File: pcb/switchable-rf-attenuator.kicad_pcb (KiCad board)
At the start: 4 copper layers, 47.4 x 31.5 mm, 26 parts, among them J1 USB_B_Mini, J2 Conn_Coaxial, J3 Conn_Coaxial, SW1 SW_SPDT, U1 AS183-73LF, U2 AS183-73LF

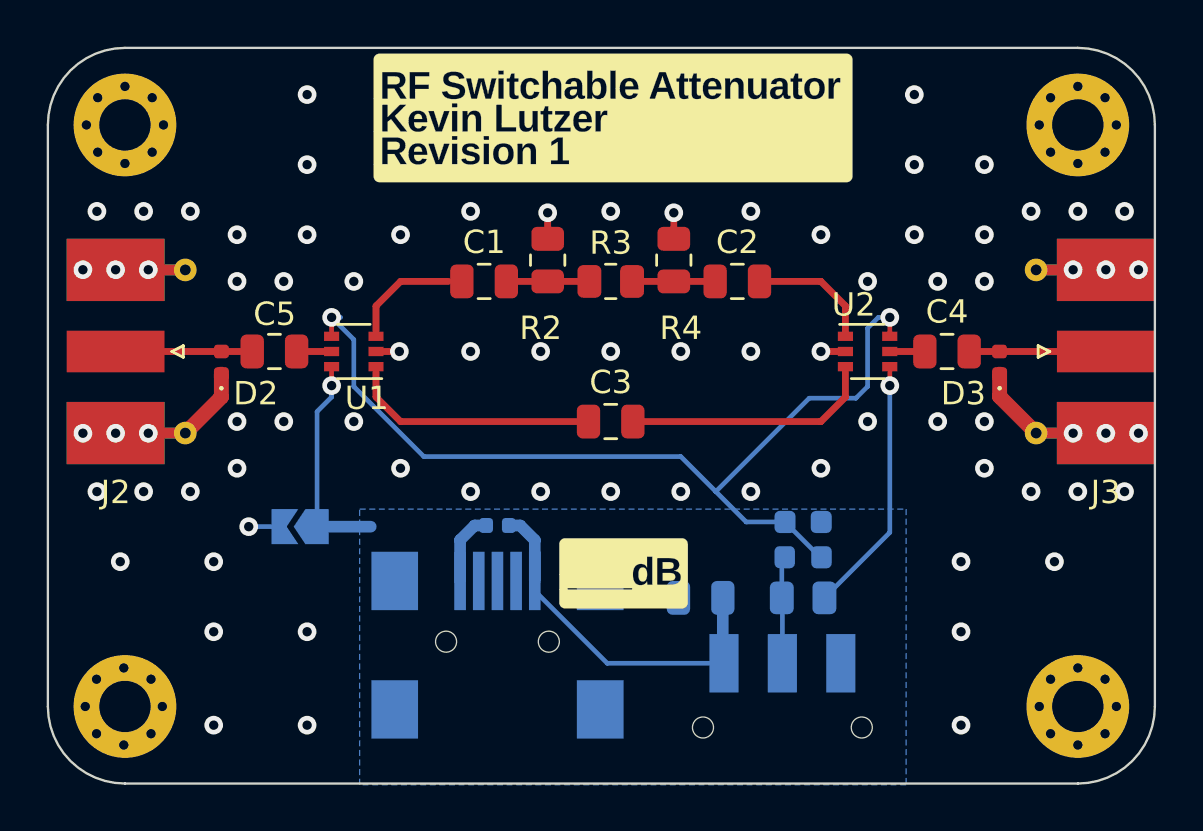
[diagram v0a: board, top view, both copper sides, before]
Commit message: WIP
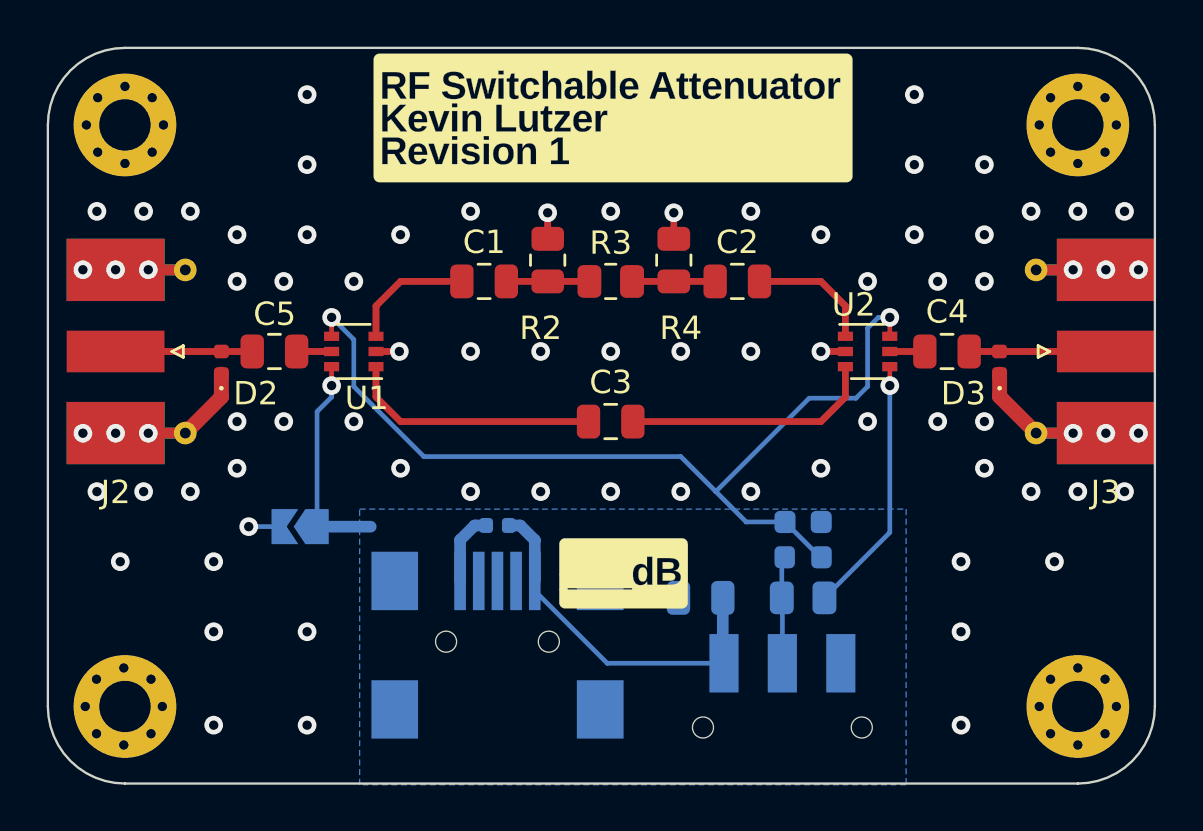
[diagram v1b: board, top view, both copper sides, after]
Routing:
- net GND: track 24.3 -> 23.6 mm
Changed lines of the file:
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@@
       (layerselection 0x00010fc_ffffffff)
       (disableapertmacros false)
-      (usegerberextensions false)
-      (usegerberattributes true)
-      (usegerberadvancedattributes true)
-      (creategerberjobfile true)
+      (usegerberextensions true)
+      (usegerberattributes false)
+      (usegerberadvancedattributes false)
+      (creategerberjobfile false)
       (svguseinch false)
       (svgprecision 6)
@@
       (plotinvisibletext false)
       (sketchpadsonfab false)
-      (subtractmaskfromsilk false)
+      (subtractmaskfromsilk true)
       (outputformat 1)
       (mirror false)
-      (drillshape 1)
+      (drillshape 0)
       (scaleselection 1)
-      (outputdirectory "")
+      (outputdirectory "../../../gerbers_v1/")
     )
   )
@@
     (fp_line (start 1 0.625) (end -1 0.625) (layer "F.Fab") (width 0.1))
     (fp_line (start 1 -0.625) (end 1 0.625) (layer "F.Fab") (width 0.1))
-    (pad "1" smd roundrect (at -0.9125 0 270) (size 1.025 1.4) (layers "F.Cu" "F.Paste" "F.Mask") (roundrect_rratio 0.243902)
+    (pad "1" smd roundrect (at -0.9125 0 270) (size 1.025 1.4) (layers "F.Cu" "F.Paste" "F.Mask") (roundrect_rratio 0.243902439)
       (net 11 "GNDA") (pintype "passive"))
-    (pad "2" smd roundrect (at 0.9125 0 270) (size 1.025 1.4) (layers "F.Cu" "F.Paste" "F.Mask") (roundrect_rratio 0.243902)
+    (pad "2" smd roundrect (at 0.9125 0 270) (size 1.025 1.4) (layers "F.Cu" "F.Paste" "F.Mask") (roundrect_rratio 0.243902439)
       (net 12 "Net-(C1-Pad2)") (pintype "passive"))
     (model "${KICAD6_3DMODEL_DIR}/Resistor_SMD.3dshapes/R_0805_2012Metric.wrl"
@@
     (fp_line (start -1 -0.625) (end 1 -0.625) (layer "F.Fab") (width 0.1))
     (fp_line (start 1 -0.625) (end 1 0.625) (layer "F.Fab") (width 0.1))
-    (pad "1" smd roundrect (at -0.9125 0) (size 1.025 1.4) (layers "F.Cu" "F.Paste" "F.Mask") (roundrect_rratio 0.243902)
+    (pad "1" smd roundrect (at -0.9125 0) (size 1.025 1.4) (layers "F.Cu" "F.Paste" "F.Mask") (roundrect_rratio 0.243902439)
       (net 12 "Net-(C1-Pad2)") (pintype "passive"))
-    (pad "2" smd roundrect (at 0.9125 0) (size 1.025 1.4) (layers "F.Cu" "F.Paste" "F.Mask") (roundrect_rratio 0.243902)
+    (pad "2" smd roundrect (at 0.9125 0) (size 1.025 1.4) (layers "F.Cu" "F.Paste" "F.Mask") (roundrect_rratio 0.243902439)
       (net 13 "Net-(C2-Pad1)") (pintype "passive"))
     (model "${KICAD6_3DMODEL_DIR}/Resistor_SMD.3dshapes/R_0805_2012Metric.wrl"
@@
     (fp_line (start 1 -0.625) (end 1 0.625) (layer "F.Fab") (width 0.1))
     (fp_line (start -1 0.625) (end -1 -0.625) (layer "F.Fab") (width 0.1))
-    (pad "1" smd roundrect (at -0.9125 0 270) (size 1.025 1.4) (layers "F.Cu" "F.Paste" "F.Mask") (roundrect_rratio 0.243902)
+    (pad "1" smd roundrect (at -0.9125 0 270) (size 1.025 1.4) (layers "F.Cu" "F.Paste" "F.Mask") (roundrect_rratio 0.243902439)
       (net 11 "GNDA") (pintype "passive"))
-    (pad "2" smd roundrect (at 0.9125 0 270) (size 1.025 1.4) (layers "F.Cu" "F.Paste" "F.Mask") (roundrect_rratio 0.243902)
+    (pad "2" smd roundrect (at 0.9125 0 270) (size 1.025 1.4) (layers "F.Cu" "F.Paste" "F.Mask") (roundrect_rratio 0.243902439)
       (net 13 "Net-(C2-Pad1)") (pintype "passive"))
     (model "${KICAD6_3DMODEL_DIR}/Resistor_SMD.3dshapes/R_0805_2012Metric.wrl"
@@
     (fp_line (start -1 0.625) (end 1 0.625) (layer "B.Fab") (width 0.1))
     (fp_line (start 1 0.625) (end 1 -0.625) (layer "B.Fab") (width 0.1))
-    (pad "1" smd roundrect (at -0.9125 0 180) (size 1.025 1.4) (layers "B.Cu" "B.Paste" "B.Mask") (roundrect_rratio 0.243902)
+    (pad "1" smd roundrect (at -0.9125 0 180) (size 1.025 1.4) (layers "B.Cu" "B.Paste" "B.Mask") (roundrect_rratio 0.243902439)
       (net 1 "GND") (pintype "passive"))
-    (pad "2" smd roundrect (at 0.9125 0 180) (size 1.025 1.4) (layers "B.Cu" "B.Paste" "B.Mask") (roundrect_rratio 0.243902)
+    (pad "2" smd roundrect (at 0.9125 0 180) (size 1.025 1.4) (layers "B.Cu" "B.Paste" "B.Mask") (roundrect_rratio 0.243902439)
       (net 18 "/V_SW") (pintype "passive"))
     (model "${KICAD6_3DMODEL_DIR}/Resistor_SMD.3dshapes/R_0805_2012Metric.wrl"
@@
   (segment (start 157.05 119.95) (end 156.425 120.575) (width 0.2) (layer "B.Cu") (net 1))
   (segment (start 156.425 125.5) (end 158.725 125.5) (width 0.5) (layer "B.Cu") (net 1))
-  (segment (start 159.275 127.35) (end 159.75 127.825) (width 0.5) (layer "B.Cu") (net 1))
   (segment (start 156.425 120.575) (end 156.425 125.5) (width 0.2) (layer "B.Cu") (net 1))
   (segment (start 180.95 125.75) (end 178.15 128.55) (width 0.2) (layer "B.Cu") (net 1))
@@
   (segment (start 165.125 125.45) (end 165.75 126.075) (width 0.5) (layer "B.Cu") (net 2))
   (segment (start 165.75 128.25) (end 165.75 127.825) (width 0.2) (layer "B.Cu") (net 2))
-  (segment (start 173.8 131.45) (end 173.85 131.5) (width 0.5) (layer "B.Cu") (net 2))
   (segment (start 168.85 131.35) (end 165.75 128.25) (width 0.2) (layer "B.Cu") (net 2))
   (segment (start 165.75 126.075) (end 165.75 127.825) (width 0.5) (layer "B.Cu") (net 2))
@@
   (segment (start 172 122.5) (end 161 122.5) (width 0.2) (layer "B.Cu") (net 3))
   (segment (start 180 117) (end 180.46 116.54) (width 0.2) (layer "B.Cu") (net 3))
-  (segment (start 157.05 116.54) (end 157.44 116.54) (width 0.2) (layer "B.Cu") (net 3))
   (segment (start 179.5 120) (end 180 119.5) (width 0.2) (layer "B.Cu") (net 3))
   (segment (start 161 122.5) (end 158 119.5) (width 0.2) (layer "B.Cu") (net 3))
